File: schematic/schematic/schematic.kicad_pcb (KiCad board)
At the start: 2 copper layers, 61 x 44 mm, 112 parts, among them IC1 DRV8830, J1 Conn_01x03, J10 Conn_01x01, J11 Conn_01x01, J12 Conn_01x01, J13 Conn_01x01, J14 Conn_01x02, J15 Conn_01x02, J2 USB_B_Micro, J3 Conn_GPIO, J4 Conn_M5StickV, J5 Conn_I2C, J6 Conn_Tale, J7 Conn_Tale, J8 Conn_01x05, J9 Conn_01x01, M1 M_Small, Q1 IRLML6402, Q2 SS8050, Q3 SS8050, Q4 PJE260N02, Q5 IRLML6402, Q6 PJE260N02, Q7 PJE260N02, Q8 BSS138, Q9 BSS138, SW1 SW_EN, SW2 SW_IO0, SW3 SW_SPDT, U1 TPS63002, U2 MPU-9250, U3 MCP73831-5-OT, U4 TPS63001, U5 FT231XS, U6 TPS63001, U7 INA219AIDCNR, U8 ESP32-WROOM-32D_GND_39

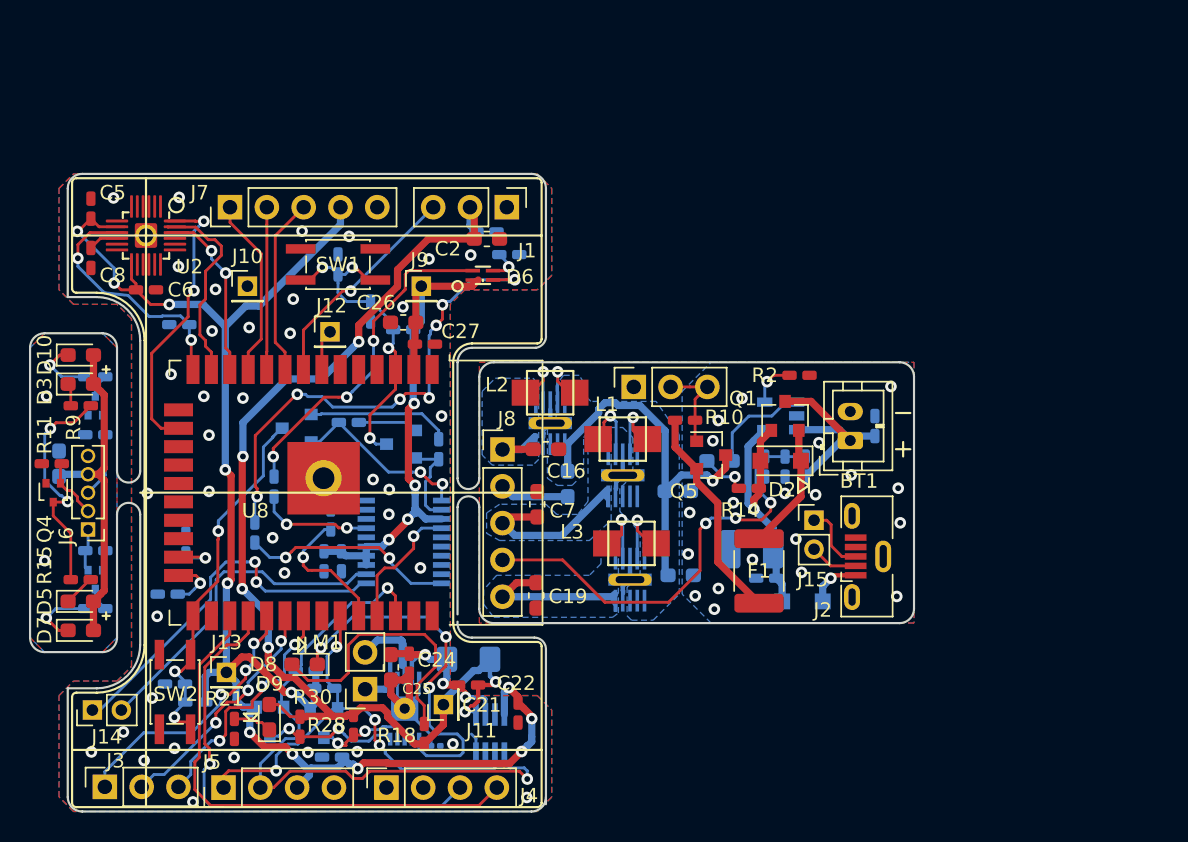
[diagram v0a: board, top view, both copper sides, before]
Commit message: Update
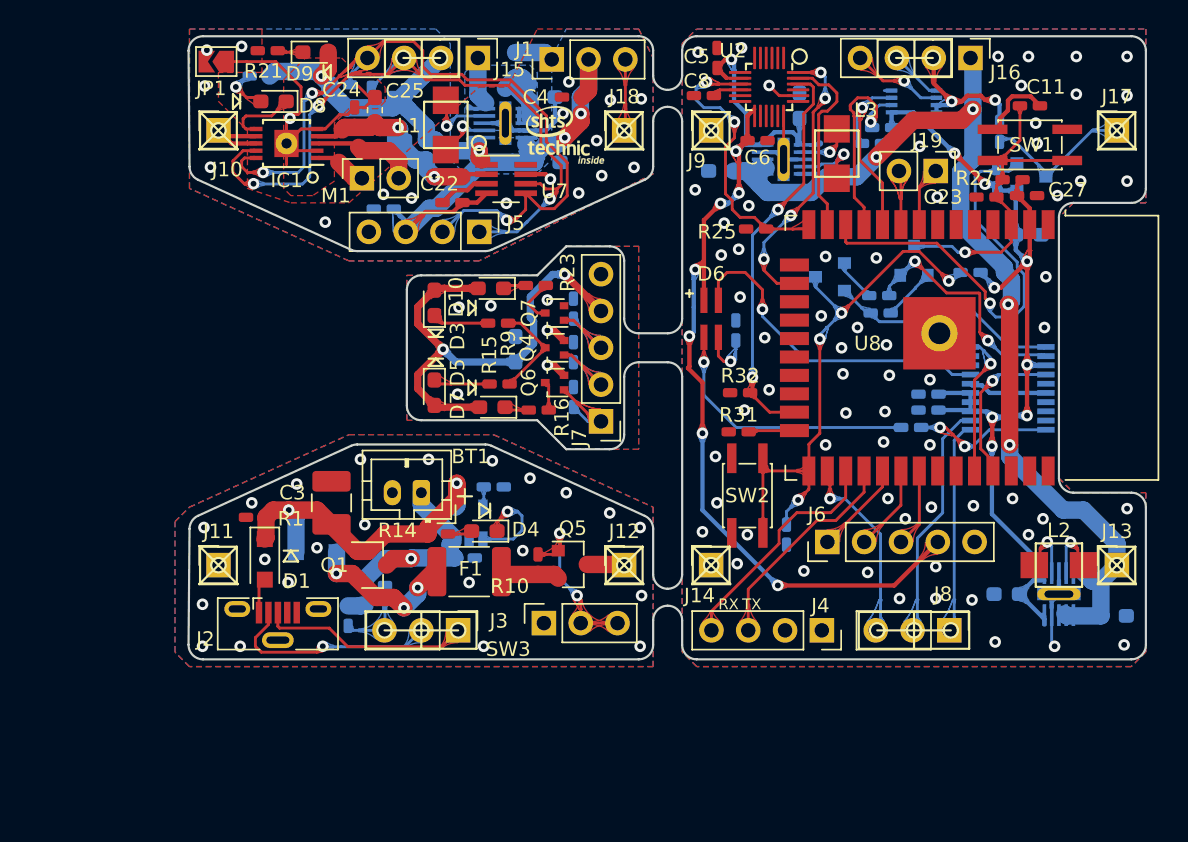
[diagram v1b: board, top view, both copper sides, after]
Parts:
- removed Q9: BSS138, Package_TO_SOT_SMD:SOT-23
- added J16: Conn_01x04, Connector_PinHeader_2.54mm:PinHeader_1x04_P2.54mm_Vertical, F.Cu at (107.9, 60.0)
- added J17: Conn_01x01, Connector_PinHeader_2.54mm:PinHeader_1x01_P2.54mm_Vertical, F.Cu at (118.0, 65.0)
- added J18: Conn_01x01, Connector_PinHeader_2.54mm:PinHeader_1x01_P2.54mm_Vertical, F.Cu at (84.0, 65.0)
- added J19: Conn_01x02, Connector_PinHeader_2.54mm:PinHeader_1x02_P2.54mm_Vertical, F.Cu at (105.5, 67.8)
- added R8: 10k, micelib:R_0402_1005Metric_HandSoldering, B.Cu at (109.9, 65.1)
- added U9: PCA9306DC, Package_SO:VSSOP-8_2.3x2mm_P0.5mm, B.Cu at (104.0, 63.0)
- C11, C23, C3, C4, D1, D4, G***, IC1, Q6, Q7, R1, R16, R23, R25, R27, R31, R32, U7: moved to F.Cu
- C16, C19, C2, C21, C26, C7, D2, R11, R18, R2, R28, R30: moved to B.Cu
- D6: value LTSN-B32JEGBB6 -> OSTB0603C1C-A; footprint micelib:LTSN-B32JEGBB6 -> micelib:OSTB0603C1C-A
- J10, J11, J12, J13, J9: footprint Connector_PinHeader_2.00mm:PinHeader_1x01_P2.00mm_Vertical -> Connector_PinHeader_2.54mm:PinHeader_1x01_P2.54mm_Vertical
- J14: value Conn_01x02 -> Conn_01x01; footprint Connector_PinHeader_2.00mm:PinHeader_1x02_P2.00mm_Vertical -> Connector_PinHeader_2.54mm:PinHeader_1x01_P2.54mm_Vertical
- J15: value Conn_01x02 -> Conn_01x04; footprint Connector_PinHeader_2.00mm:PinHeader_1x02_P2.00mm_Vertical -> Connector_PinHeader_2.54mm:PinHeader_1x04_P2.54mm_Vertical
- J3: value Conn_GPIO -> Conn_01x03; footprint Connector_PinSocket_2.54mm:PinSocket_1x03_P2.54mm_Vertical -> Connector_PinHeader_2.54mm:PinHeader_1x03_P2.54mm_Vertical
- J6: footprint Connector_PinHeader_1.27mm:PinHeader_1x05_P1.27mm_Vertical -> Connector_PinHeader_2.54mm:PinHeader_1x05_P2.54mm_Vertical
- J8: value Conn_01x05 -> Conn_01x03; footprint Connector_PinHeader_2.54mm:PinHeader_1x05_P2.54mm_Vertical -> Connector_PinHeader_2.54mm:PinHeader_1x03_P2.54mm_Vertical
- JP1: footprint Resistor_SMD:R_0201_0603Metric -> Jumper:SolderJumper-2_P1.3mm_Open_TrianglePad1.0x1.5mm; moved to F.Cu
- R7: value 470 -> 10k; footprint micelib:C_0402_1005Metric_HandSoldering -> micelib:R_0402_1005Metric_HandSoldering
- moved J13 61.9 mm to (118.0, 95.0)
- moved Q8 61.7 mm to (112.1, 68.2), turned to 0 degrees
- moved R29 61.2 mm to (107.9, 74.8)
- moved R24 54.6 mm to (101.8, 64.8)
- moved R26 53.3 mm to (101.1, 65.9), turned to 180 degrees
- moved R7 51.6 mm to (109.7, 68.3), turned to 270 degrees
- moved J6 51.0 mm to (98.0, 93.4), turned to 90 degrees
- moved JP1 49.6 mm to (55.9, 60.2), turned to 180 degrees
- moved C11 49.0 mm to (112.0, 63.3), turned to 0 degrees
- moved SW1 48.5 mm to (112.0, 66.0)
- moved R21 46.9 mm to (59.4, 59.5), turned to 180 degrees
- moved R18 46.8 mm to (58.9, 61.2), turned to 180 degrees
- moved D9 46.0 mm to (62.7, 59.6), turned to 0 degrees
- moved R20 46.0 mm to (105.0, 80.9), turned to 180 degrees
- moved R12 45.9 mm to (103.8, 85.5), turned to 180 degrees
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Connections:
- C18 pad 1: +3V3 -> +5V
- C22 pad 1: +3V3 -> +5V
- D6 pad 1: +3.3VA -> +3V3
- J1 pad 3: PWM0 -> PWM0_5V
- J11 pad 1: +5V -> GNDD
- J12 pad 1: ADC1_Batt -> +BATT
- J13 pad 1: +3V3 -> +BATT
- J14 pad 1: D+ -> GNDD
- J15 pad 1: D+ -> +BATT
- J15 pad 2: D- -> +5V
- J3 pad 1: GPIO_5 -> D+
- J3 pad 2: GPIO_18 -> D-
- J3 pad 3: GPIO_19 -> ADC1_Batt
- J5 pad 1: I2C_SDA -> I2C_SDA_5V
- J5 pad 2: I2C_SCL -> I2C_SCL_5V
- J5 pad 3: +3V3 -> +5V
- J8 pad 1: +3.3VA -> D+
- J8 pad 2: GNDD -> D-
- J8 pad 3: +5V -> ADC1_Batt
- J9 pad 1: +3.3VA -> GNDD
- Q8 pad 1: +3V3 -> +3.3VA
- Q8 pad 2: I2C_SDA -> PWM0
- Q8 pad 3: I2C_SDA_5V -> PWM0_5V
- R12 pad 2: Net-(D6-Pad2) -> Net-(D6-Pad3)
- R13 pad 1: Net-(D6-Pad3) -> Net-(D6-Pad4)
- R20 pad 2: Net-(D6-Pad4) -> Net-(D6-Pad2)
- R24 pad 2: +3V3 -> +3.3VA
- R26 pad 1: +3V3 -> +3.3VA
- R29 pad 1: +3V3 -> +3.3VA
- R32 pad 2: Net-(R32-Pad2) -> IMU_CS
- R7 pad 1: UART_RX -> PWM0
- R7 pad 2: Net-(R7-Pad2) -> +3.3VA
- U5 pad 20: Net-(R7-Pad2) -> UART_RX
- U7 pad 4: +3V3 -> +5V
- U7 pad 5: I2C_SCL -> I2C_SCL_5V
- U7 pad 6: I2C_SDA -> I2C_SDA_5V
- U8 pad 10: LED_BRAKE -> I2C_SDA
- U8 pad 11: LED_RIGHT -> I2C_SCL
- U8 pad 12: IMU_CS -> PWM0
- U8 pad 23: Net-(R32-Pad2) -> IMU_CS
- U8 pad 26: (no net) -> ADC1_Batt
- U8 pad 29: GPIO_5 -> LED_RIGHT
- U8 pad 30: GPIO_18 -> LED_BRAKE
- U8 pad 31: GPIO_19 -> LED_LEFT
- U8 pad 33: I2C_SDA -> (no net)
- U8 pad 36: I2C_SCL -> (no net)
- U8 pad 7: ADC1_Batt -> (no net)
- U8 pad 8: PWM0 -> GPIO_32
- U8 pad 9: LED_LEFT -> GPIO_33
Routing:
- net +BATT: track 26.9 -> 85.7 mm, vias 1 -> 4
- net I2C_SCL_5V: track 9.72 -> 59.0 mm, vias 2 -> 4
- net I2C_SDA_5V: track 7.22 -> 54.7 mm, vias 2 -> 3
- net GNDD: track 12.6 -> 48.2 mm, vias 60 -> 109
- net +3V3: track 139.3 -> 106.0 mm, vias 12 -> 10
- net I2C_SCL: track 44.3 -> 15.1 mm, vias 2 -> 1
- net +3.3VA: track 41.9 -> 68.1 mm, vias 4 -> 8
- net FAULTn: track 25.7 -> 4.95 mm, vias 3 -> 0
- net I2C_SDA: track 33.7 -> 13.8 mm, vias 4 -> 1
- net Net-(D6-Pad4): track 23.8 -> 4.02 mm, vias 3 -> 1
- net GPIO_5: track 18.8 -> 0.00 mm, vias 3 -> 0
- net ESP32_RX: track 34.8 -> 16.2 mm
- net ESP32_TX: track 32.9 -> 15.1 mm, vias 1 -> 0
- net GPIO_19: track 17.1 -> 0.00 mm, vias 3 -> 0
- net GPIO_18: track 16.7 -> 0.00 mm, vias 3 -> 0
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- added copper zone on F.Cu, net GND
- removed copper zone on B.Cu, net +3.3VA
- removed copper zone on B.Cu, net +3V3
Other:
- board size 61 x 44 mm -> 66.1 x 43 mm
- net class PowerBroad added: clearance 0.18, trace_width 1.2, via_dia 0.8, via_drill 0.4
- net class PowerMiddle added: clearance 0.18, trace_width 0.5, via_dia 0.8, via_drill 0.4
- net class PowerNarrow added: clearance 0.18, trace_width 0.2, via_dia 0.8, via_drill 0.4
- net class Power_broad removed
- net class Power_narrow removed
- board text added: "RX"
- board text added: "TX"
